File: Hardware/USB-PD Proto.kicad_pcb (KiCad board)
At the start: 2 copper layers, 34 x 34 mm, 12 parts, among them J2 Conn_01x04_Male, J3 Conn_01x02_Male, J4 Conn_01x02_Male, J5 Conn_01x02_Male, J6 Conn_01x02_Male, J7 Conn_01x08_Male

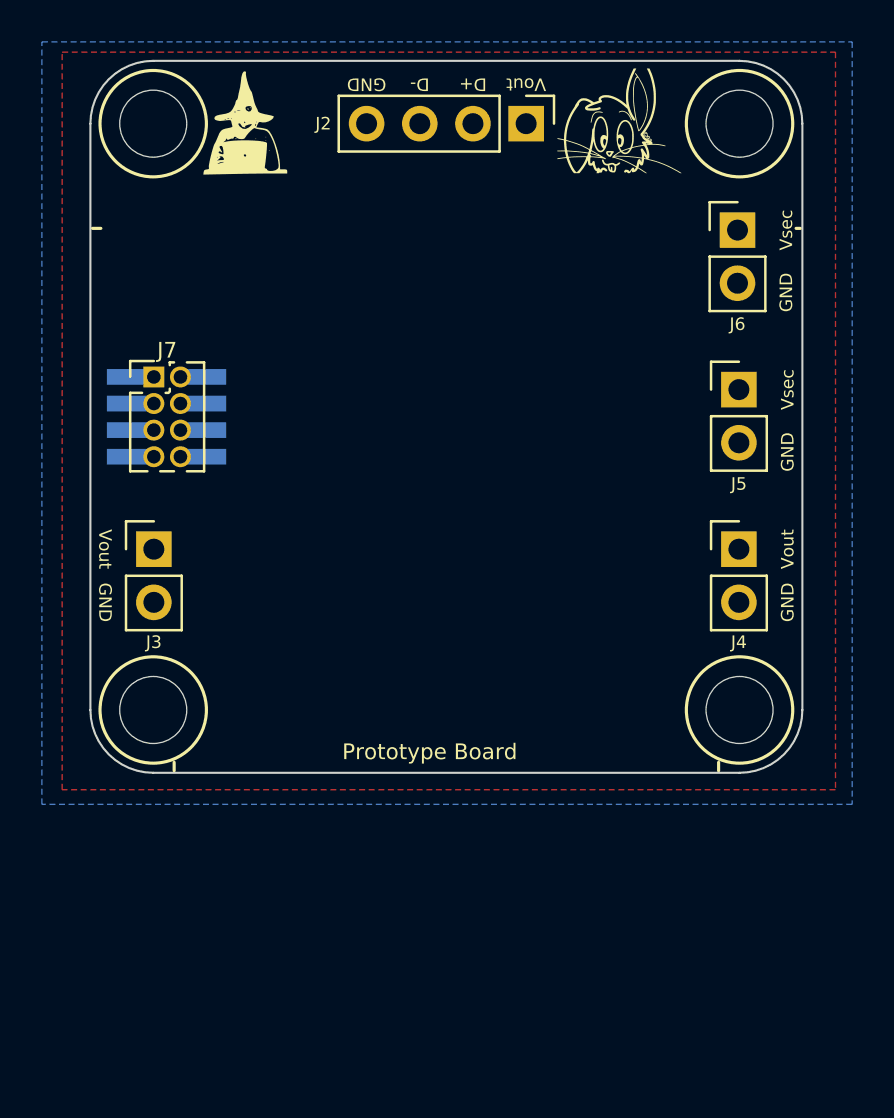
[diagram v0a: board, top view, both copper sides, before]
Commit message: Uber Rework!
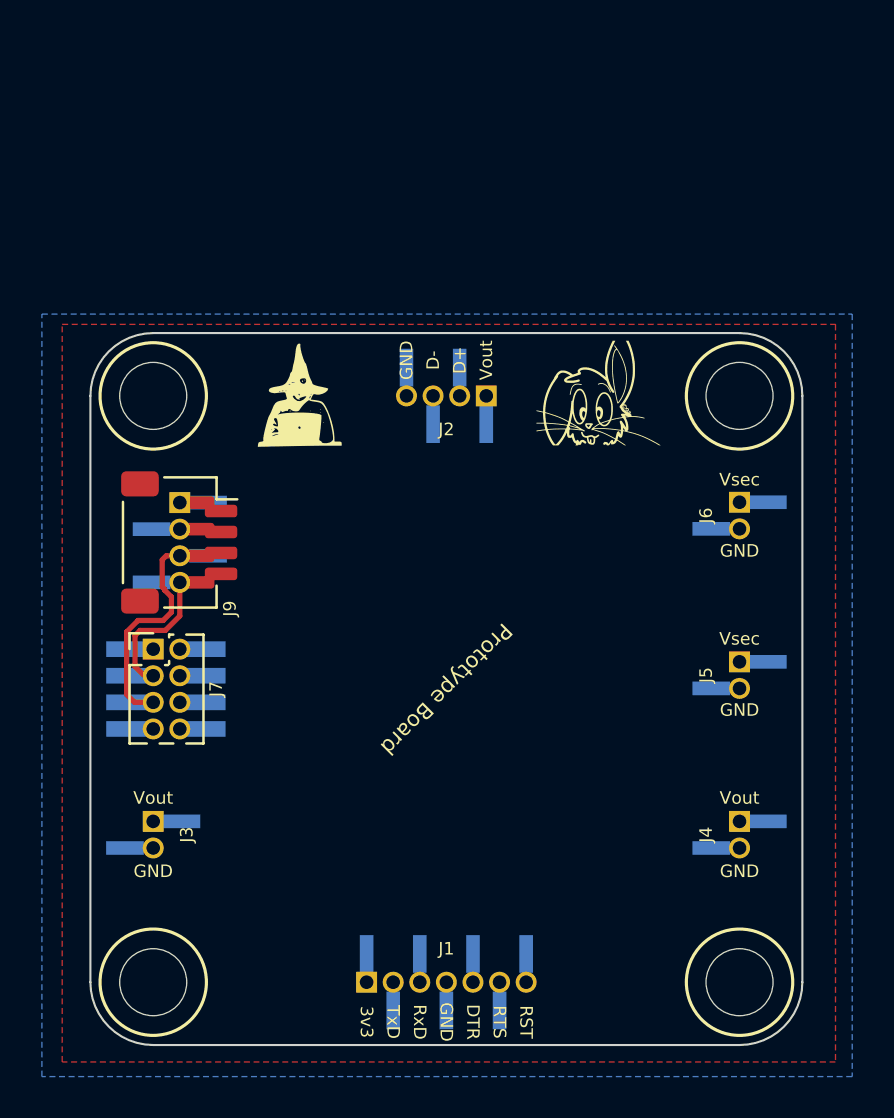
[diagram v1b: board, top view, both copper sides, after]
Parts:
- added J1: Conn_01x07_Male, Tinker:Board_Stacker_7, F.Cu at (96.2, 114.0)
- added J9: QWIIC_Stackable, Tinker:QWIIC_Stack_II, F.Cu at (87.3, 93.0)
- J2: footprint Tinker:PinHeader_1x04_P2.54mm_Vertical -> Tinker:Board_Stacker_4
- J3, J4, J5, J6: footprint Tinker:PinHeader_1x02_P2.54mm_Vertical -> Tinker:Board_Stacker_2
- moved G*** 13.3 mm to (93.0, 85.9)
- moved J2 13.1 mm to (101.9, 86.0)
- moved REF** 13.0 mm to (107.0, 86.5)
- moved J6 13.0 mm to (114.0, 91.1)
- moved J3 13.0 mm to (86.0, 106.3)
- moved J4 13.0 mm to (114.0, 106.3)
- moved J5 13.0 mm to (114.0, 98.7)
- moved J7 13.0 mm to (86.0, 98.1)
- moved REF** 13.0 mm to (114.0, 114.0)
- moved REF** 13.0 mm to (86.0, 114.0)
- moved REF** 13.0 mm to (114.0, 86.0)
- moved REF** 13.0 mm to (86.0, 86.0)
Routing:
- net SDA: track 0.00 -> 10.6 mm
- net SCL: track 0.00 -> 6.15 mm
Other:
- board text added: "3v3"
- board text added: "DTR"
- board text added: "RST"
- board text added: "RTS"
- board text added: "RxD"
- board text added: "TxD"
